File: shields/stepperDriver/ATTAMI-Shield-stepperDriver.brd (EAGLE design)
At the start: 22.5 x 30.5 mm, 15 parts

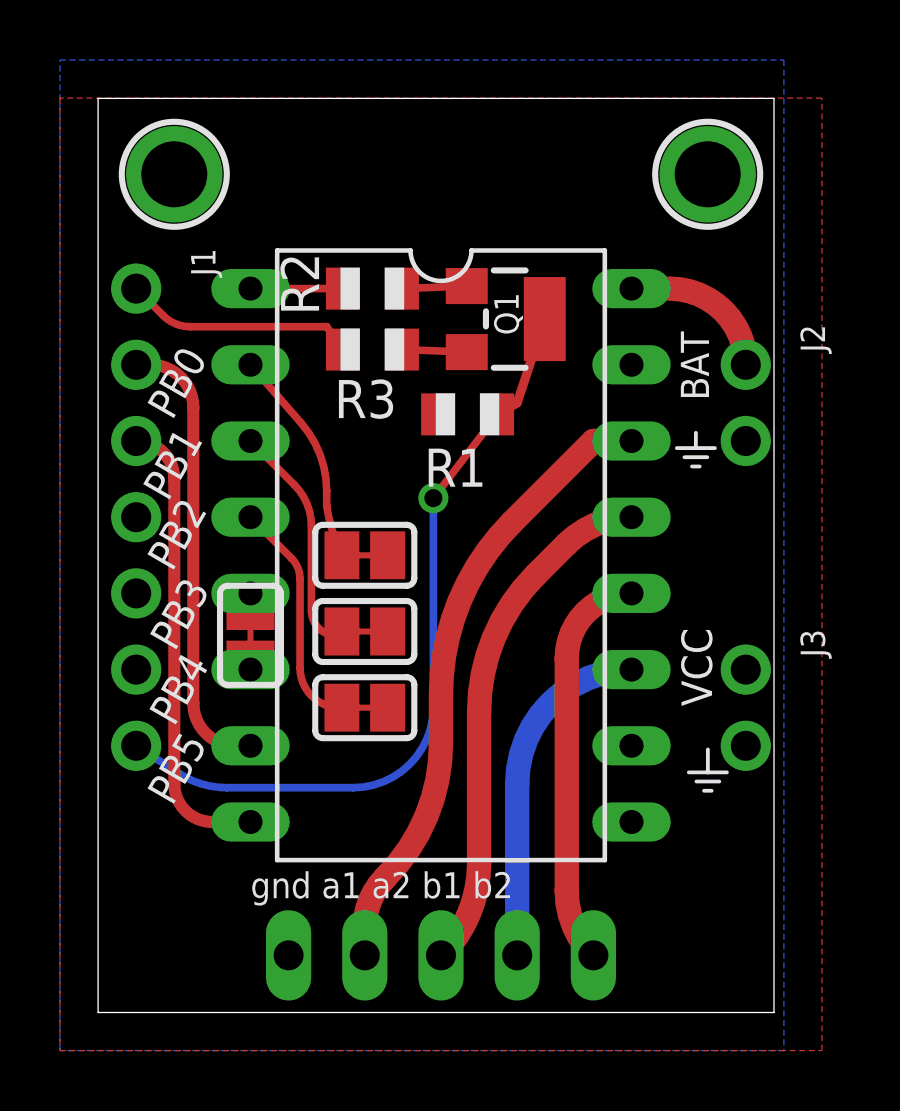
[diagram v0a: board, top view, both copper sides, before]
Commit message: updtae A4988 lib part
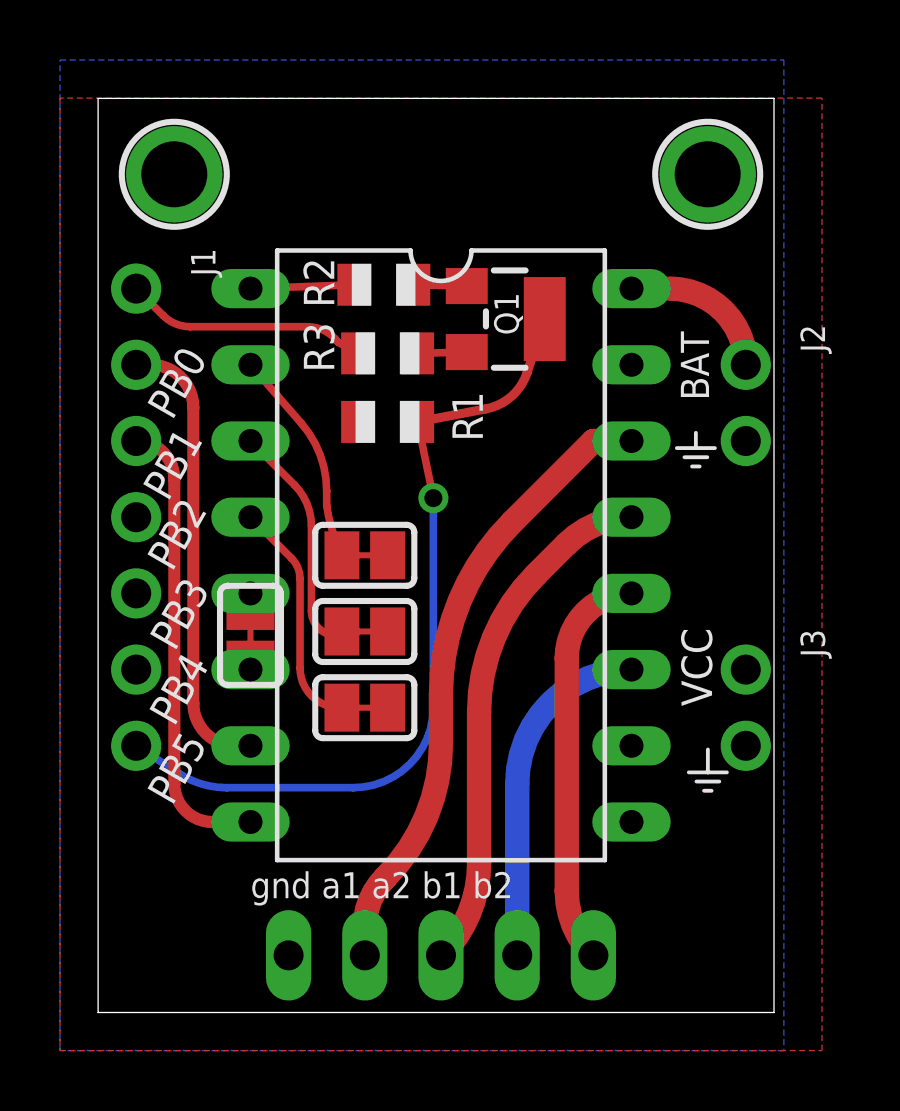
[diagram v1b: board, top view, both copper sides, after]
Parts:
- BRK1: value STEPPER_driver -> A4988_driver
- moved R1 2.68 mm to (9.65, 19.7)
- moved R3 0.52 mm to (9.65, 22.0)
- moved R2 0.40 mm to (9.53, 24.3)
- renumbered U$3 to BRK1
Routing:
- net PB5: track 25.5 -> 27.0 mm
- net N$4: track 2.15 -> 1.64 mm
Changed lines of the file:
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@@
 <attribute name="VALUE" x="12.954" y="21.082" size="0.4064" layer="27" ratio="10" rot="R270"/>
 </element>
-<element name="R1" library="adafruit" package="R0805" value="" x="12.319" y="19.939" smashed="yes">
-<attribute name="NAME" x="12.954" y="18.796" size="1.27" layer="25" rot="R180"/>
-<attribute name="VALUE" x="11.557" y="17.653" size="1.27" layer="27"/>
-</element>
-<element name="R2" library="adafruit" package="R0805" value="" x="9.144" y="24.13" smashed="yes">
-<attribute name="NAME" x="7.366" y="23.241" size="1.27" layer="25" rot="R90"/>
-<attribute name="VALUE" x="8.382" y="21.844" size="1.27" layer="27"/>
-</element>
-<element name="R3" library="adafruit" package="R0805" value="" x="9.144" y="22.098" smashed="yes">
-<attribute name="NAME" x="7.874" y="19.812" size="1.27" layer="25"/>
-<attribute name="VALUE" x="8.382" y="19.812" size="1.27" layer="27"/>
+<element name="R1" library="adafruit" package="R0805" value="" x="9.652" y="19.685" smashed="yes">
+<attribute name="NAME" x="11.811" y="20.701" size="1.016" layer="25" rot="R270"/>
+<attribute name="VALUE" x="8.89" y="17.399" size="1.27" layer="27"/>
+</element>
+<element name="R2" library="adafruit" package="R0805" value="" x="9.525" y="24.257" smashed="yes">
+<attribute name="NAME" x="7.874" y="23.495" size="1.016" layer="25" rot="R90"/>
+<attribute name="VALUE" x="8.763" y="21.971" size="1.27" layer="27"/>
+</element>
+<element name="R3" library="adafruit" package="R0805" value="" x="9.652" y="21.971" smashed="yes">
+<attribute name="NAME" x="7.874" y="21.336" size="1.016" layer="25" rot="R90"/>
+<attribute name="VALUE" x="8.89" y="19.685" size="1.27" layer="27"/>
 </element>
 <element name="SJ1" library="microbuilder" package="SOLDERJUMPER_CLOSEDWIRE" value="" x="8.89" y="10.16" smashed="yes" rot="R180">
@@
 <element name="U$1" library="microbuilder" package="MOUNTINGHOLE_2.0_PLATED" value="MOUNTINGHOLE2.0" x="20.32" y="27.94"/>
 <element name="U$2" library="microbuilder" package="MOUNTINGHOLE_2.0_PLATED" value="MOUNTINGHOLE2.0" x="2.54" y="27.94"/>
-<element name="U$3" library="ATtami" package="DIL16" value="STEPPER_driver" x="11.43" y="15.24" smashed="yes">
+<element name="BRK1" library="ATtami" package="DIL16" value="A4988_driver" x="11.43" y="15.24" smashed="yes">
 <attribute name="VALUE" x="15.875" y="5.334" size="1.27" layer="27" ratio="10" rot="R90"/>
 </element>
@@
 <contactref element="J1" pad="1"/>
 <contactref element="R3" pad="1"/>
-<contactref element="U$3" pad="16"/>
+<contactref element="BRK1" pad="16"/>
 <polygon width="0.4064" layer="16">
 <vertex x="-1.27" y="31.75"/>
@@
 <vertex x="-1.27" y="-1.27"/>
 </polygon>
-<wire x1="7.62" y1="22.86" x2="3.06605" y2="22.86" width="0.254" layer="1"/>
+<wire x1="3.06605" y1="22.86" x2="6.975896875" y2="22.86" width="0.254" layer="1"/>
+<wire x1="6.975896875" y1="22.86" x2="8.00054375" y2="22.34033125" width="0.254" layer="1" curve="-53.785325"/>
+<wire x1="8.00054375" y1="22.34033125" x2="8.652" y2="21.971" width="0.254" layer="1"/>
 <wire x1="3.06605" y1="22.86" x2="2.168025" y2="23.231975" width="0.254" layer="1" curve="-45"/>
 <wire x1="2.168025" y1="23.231975" x2="1.27" y2="24.13" width="0.254" layer="1"/>
-<contactref element="U$3" pad="10"/>
+<contactref element="BRK1" pad="10"/>
 <contactref element="JP1" pad="1"/>
-<wire x1="7.62" y1="22.86" x2="8.144" y2="22.098" width="0.254" layer="1"/>
 </signal>
 <signal name="VCC">
 <contactref element="J3" pad="1"/>
 <contactref element="R1" pad="1"/>
-<contactref element="U$3" pad="15"/>
+<contactref element="BRK1" pad="15"/>
 <contactref element="SJ1" pad="1"/>
 <contactref element="SJ2" pad="1"/>
@@
 <contactref element="J2" pad="1"/>
 <wire x1="19.05" y1="24.13" x2="21.59" y2="21.59" width="0.8128" layer="1" curve="-90"/>
-<contactref element="U$3" pad="9"/>
+<contactref element="BRK1" pad="9"/>
 <wire x1="17.78" y1="24.13" x2="19.05" y2="24.13" width="0" layer="19" extent="1-1"/>
 </signal>
 <signal name="PB0">
 <contactref element="J1" pad="2"/>
-<contactref element="U$3" pad="7"/>
+<contactref element="BRK1" pad="7"/>
 <wire x1="1.27" y1="21.59" x2="1.755096875" y2="21.59" width="0.4064" layer="1"/>
 <wire x1="1.755096875" y1="21.59" x2="3.175" y2="20.170096875" width="0.4064" layer="1" curve="-90"/>
@@
 <signal name="PB1">
 <contactref element="J1" pad="3"/>
-<contactref element="U$3" pad="8"/>
+<contactref element="BRK1" pad="8"/>
 <wire x1="1.27" y1="19.05" x2="2.54" y2="17.78" width="0.4064" layer="1" curve="-90"/>
 <wire x1="2.54" y1="17.78" x2="2.54" y2="7.62" width="0.4064" layer="1"/>
@@
 <contactref element="Q1" pad="3"/>
 <contactref element="J1" pad="7"/>
-<wire x1="13.319" y1="19.939" x2="11.176" y2="17.145" width="0.254" layer="1"/>
+<wire x1="10.652" y1="19.685" x2="11.176" y2="17.145" width="0.254" layer="1"/>
 <via x="11.176" y="17.145" extent="1-16" drill="0.6" shape="square"/>
 <wire x1="11.176" y1="17.145" x2="11.176" y2="10.172065625" width="0.254" layer="16"/>
@@
 <wire x1="4.292428125" y1="7.493" x2="2.704090625" y2="7.962059375" width="0.254" layer="16" curve="-32.905279"/>
 <wire x1="2.704090625" y1="7.962059375" x2="1.27" y2="8.89" width="0.254" layer="16"/>
-<wire x1="14.889" y1="23.114" x2="13.97" y2="20.32" width="0.3048" layer="1"/>
-<wire x1="13.97" y1="20.32" x2="13.319" y2="19.939" width="0.3048" layer="1"/>
+<wire x1="14.889" y1="23.114" x2="14.3002875" y2="21.324159375" width="0.3048" layer="1"/>
+<wire x1="14.3002875" y1="21.324159375" x2="12.931759375" y2="20.1213" width="0.3048" layer="1" curve="-60.958763"/>
+<wire x1="12.931759375" y1="20.1213" x2="10.652" y2="19.685" width="0.3048" layer="1"/>
 </signal>
 <signal name="N$4">
 <contactref element="R3" pad="2"/>
 <contactref element="Q1" pad="2"/>
-<wire x1="12.289" y1="22.014" x2="10.144" y2="22.098" width="0.254" layer="1"/>
+<wire x1="12.289" y1="22.014" x2="10.652" y2="21.971" width="0.254" layer="1"/>
 </signal>
 <signal name="N$5">
 <contactref element="Q1" pad="1"/>
 <contactref element="R2" pad="2"/>
-<wire x1="10.144" y1="24.13" x2="12.289" y2="24.214" width="0.254" layer="1"/>
+<wire x1="10.525" y1="24.257" x2="12.289" y2="24.214" width="0.254" layer="1"/>
 </signal>
 <signal name="ENABLE">
 <contactref element="R2" pad="1"/>
-<contactref element="U$3" pad="1"/>
-<wire x1="5.08" y1="24.13" x2="8.144" y2="24.13" width="0.254" layer="1"/>
+<contactref element="BRK1" pad="1"/>
+<wire x1="5.08" y1="24.13" x2="8.525" y2="24.257" width="0.254" layer="1"/>
 </signal>
 <signal name="N$10">
 <contactref element="SJ3" pad="2"/>
-<contactref element="U$3" pad="2"/>
+<contactref element="BRK1" pad="2"/>
 <wire x1="8.128" y1="15.24" x2="8.063171875" y2="15.434484375" width="0.254" layer="1"/>
 <wire x1="8.063171875" y1="15.434484375" x2="7.62" y2="16.89543125" width="0.254" layer="1" curve="-18.434976"/>
@@
 <signal name="N$13">
 <contactref element="SJ2" pad="2"/>
-<contactref element="U$3" pad="3"/>
+<contactref element="BRK1" pad="3"/>
 <wire x1="8.128" y1="12.7" x2="7.92519375" y2="12.573" width="0.254" layer="1"/>
 <wire x1="7.92519375" y1="12.573" x2="7.112" y2="13.38619375" width="0.254" layer="1" curve="-90"/>
@@
 <signal name="N$14">
 <contactref element="SJ1" pad="2"/>
-<contactref element="U$3" pad="4"/>
+<contactref element="BRK1" pad="4"/>
 <wire x1="5.08" y1="16.51" x2="6.4477125" y2="15.1422875" width="0.254" layer="1"/>
 <wire x1="6.4477125" y1="15.1422875" x2="6.731" y2="14.458371875" width="0.254" layer="1" curve="-45"/>
@@
 <signal name="N$3">
 <contactref element="JP1" pad="2"/>
-<contactref element="U$3" pad="11"/>
+<contactref element="BRK1" pad="11"/>
 <wire x1="17.78" y1="19.05" x2="16.51" y2="19.05" width="0.8128" layer="1"/>
 <wire x1="16.51" y1="19.05" x2="13.811796875" y2="16.351796875" width="0.8128" layer="1"/>
@@
 <signal name="N$6">
 <contactref element="JP1" pad="3"/>
-<contactref element="U$3" pad="12"/>
+<contactref element="BRK1" pad="12"/>
 <wire x1="17.78" y1="16.51" x2="15.611975" y2="15.611975" width="0.8128" layer="1" curve="45"/>
 <wire x1="15.611975" y1="15.611975" x2="14.596703125" y2="14.596703125" width="0.8128" layer="1"/>
@@
 <signal name="N$7">
 <contactref element="JP1" pad="4"/>
-<contactref element="U$3" pad="14"/>
+<contactref element="BRK1" pad="14"/>
 <wire x1="17.78" y1="11.43" x2="13.97" y2="7.62" width="0.8128" layer="16" curve="90"/>
 <wire x1="13.97" y1="7.62" x2="13.97" y2="1.905" width="0.8128" layer="16"/>
@@
 <signal name="N$8">
 <contactref element="JP1" pad="5"/>
-<contactref element="U$3" pad="13"/>
+<contactref element="BRK1" pad="13"/>
 <wire x1="17.78" y1="13.97" x2="15.621" y2="11.811" width="0.8128" layer="1" curve="90"/>
 <wire x1="15.621" y1="11.811" x2="15.621" y2="4.051234375" width="0.8128" layer="1"/>
@@
 </signal>
 <signal name="N$2">
-<contactref element="U$3" pad="5"/>
+<contactref element="BRK1" pad="5"/>
 <contactref element="SJ4" pad="2"/>
 <wire x1="5.08" y1="13.335" x2="5.08" y2="13.97" width="0.4064" layer="1"/>
@@
 <signal name="N$9">
 <contactref element="SJ4" pad="1"/>
-<contactref element="U$3" pad="6"/>
+<contactref element="BRK1" pad="6"/>
 <wire x1="5.08" y1="11.43" x2="5.08" y2="11.811" width="0.4064" layer="1"/>
 </signal>
